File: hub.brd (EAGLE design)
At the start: 160 x 100 mm, 27 parts, among them U1 10118194-MICRO-USB, U2 LM3671MF-3.3/NOPBMF05A-M, U3 SN74LVC1T45DBVRDBV6-M, U4 SN74LVC1T45DBVRDBV6-M

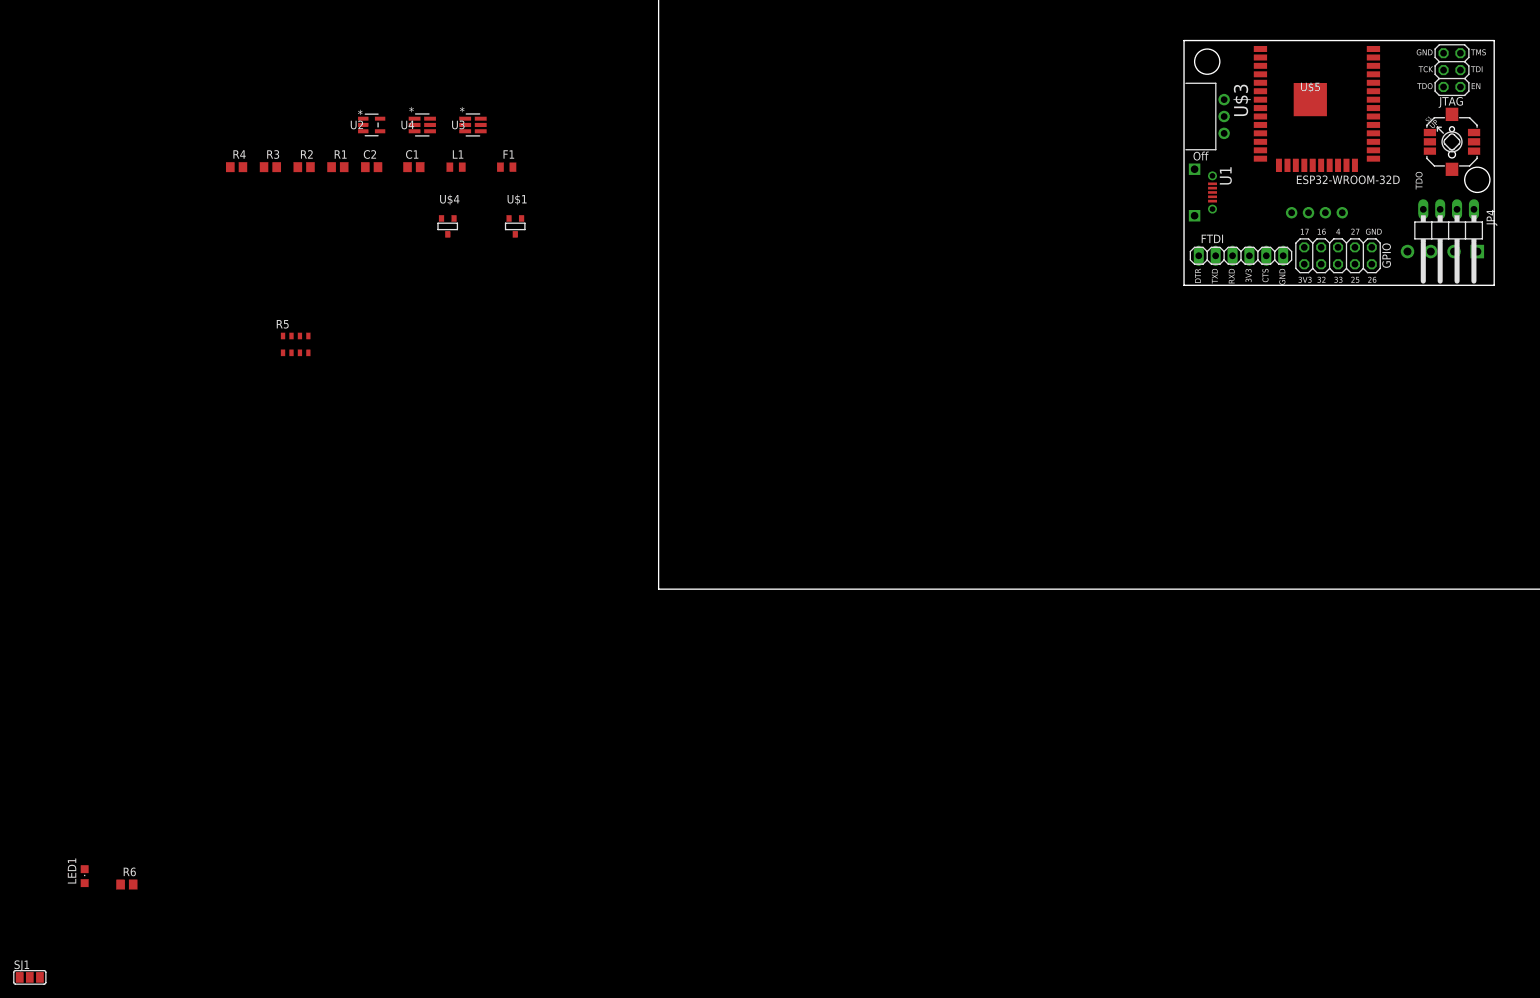
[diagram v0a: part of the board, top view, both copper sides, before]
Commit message: First draft of component layout
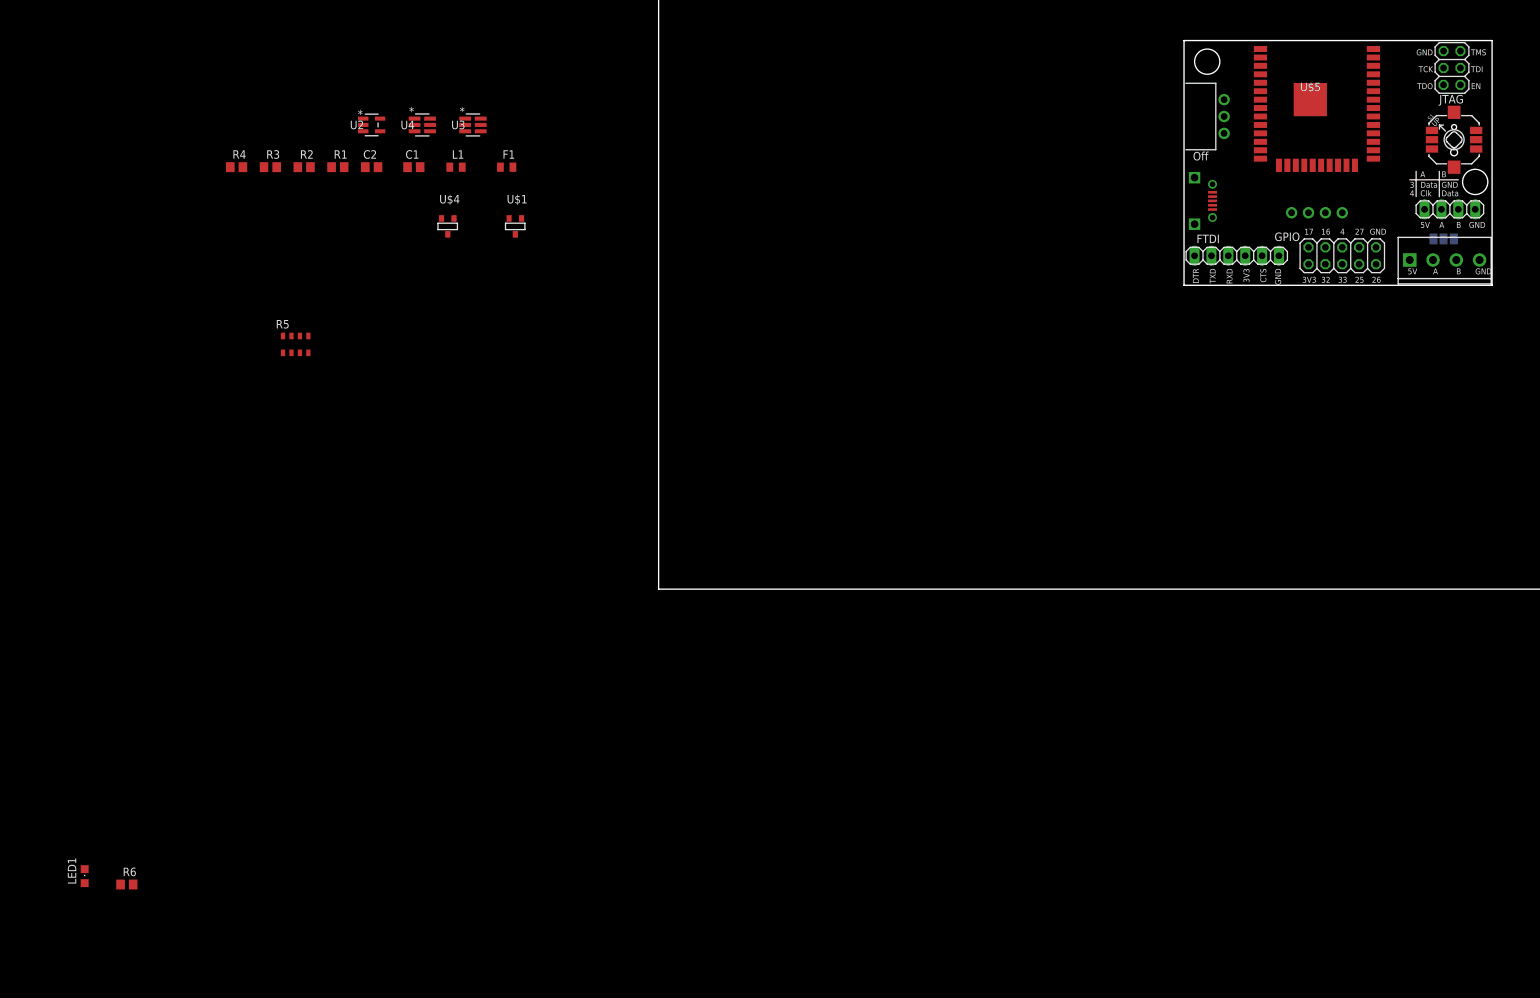
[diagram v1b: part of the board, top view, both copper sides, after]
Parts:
- removed JP4: 4-pin LED Strip, pinhead:1X04/90
- added JP1: (no value), pinhead:1X04
- moved SJ1 240.0 mm to (118.1, 52.7), flipped to the bottom
- moved J1 10.2 mm to (113.0, 49.5), flipped to the top
- moved U1 1.27 mm to (80.6, 58.4)
- moved JP7 0.64 mm to (102.9, 50.2)
- moved JP2 0.63 mm to (87.0, 50.2)
- moved S1 0.45 mm to (119.7, 67.6)
- moved JP3 0.32 mm to (119.4, 78.4)
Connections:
- net +5V: now also J1.1, JP1.1; no longer JP4.1
- net GND: now also JP1.4; no longer JP4.4
- net N$7: now also JP1.3; no longer JP4.3
- net N$9: now also JP1.2; no longer JP4.2
- net VCC: no longer J1.1
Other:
- outline, holes or cut-outs redrawn
- board text added: "3"
- board text added: "3-pin"
- board text added: "4-pin"
- board text added: "5V"
- board text added: "A"
- board text added: "B"
- board text added: "Clk"
- board text added: "Data"
